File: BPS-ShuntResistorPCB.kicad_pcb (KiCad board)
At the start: 2 copper layers, 37.6 x 32.5 mm, 7 parts, among them J1 Amp_Conn

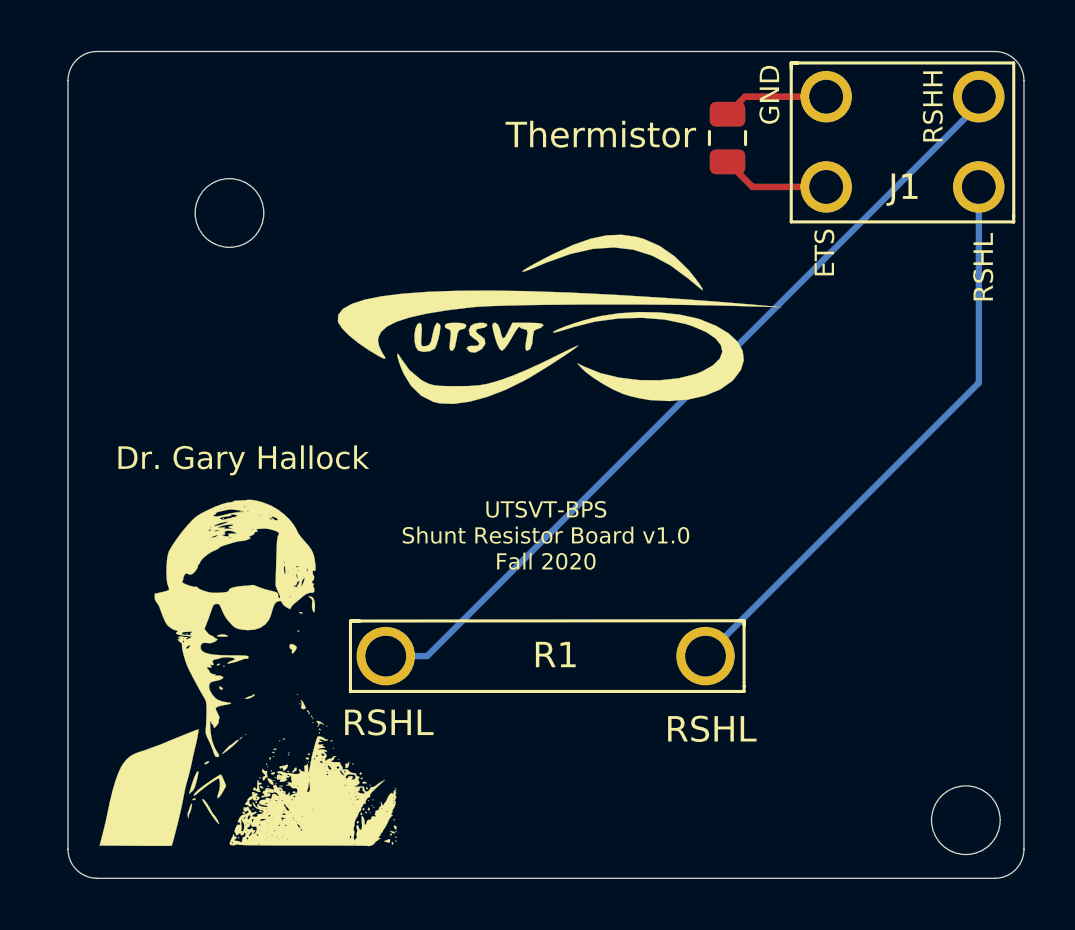
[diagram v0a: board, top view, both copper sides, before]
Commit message: fixed typo
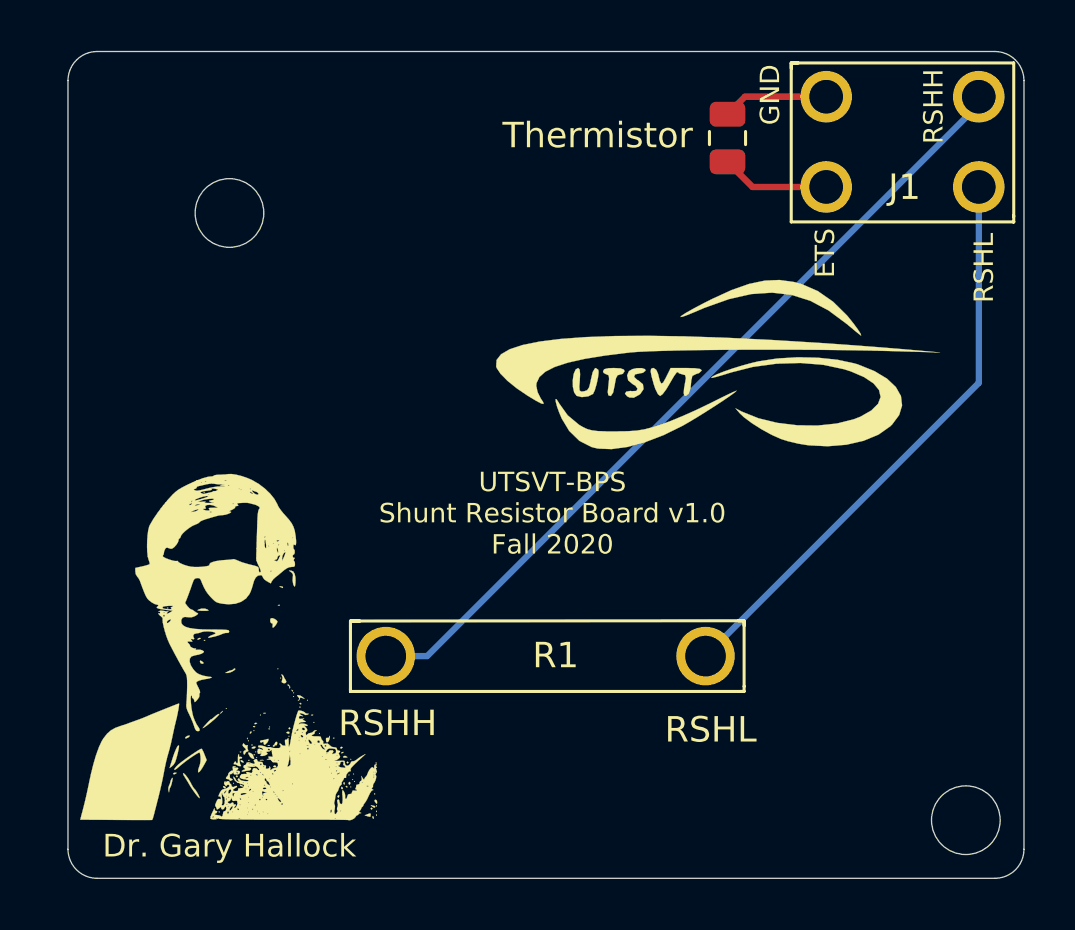
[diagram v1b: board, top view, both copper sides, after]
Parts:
- moved LOGO1 6.47 mm to (168.8, 84.7)
- moved LOGO2 1.27 mm to (149.4, 95.5)
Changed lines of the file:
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@@
     (mod_text_size 1 1)
     (mod_text_width 0.15)
-    (pad_size 2.028 2.028)
-    (pad_drill 1.328)
+    (pad_size 2.7 2.7)
+    (pad_drill 2.7)
     (pad_to_mask_clearance 0.05)
     (aux_axis_origin 0 0)
@@
       (effects (font (size 1 1) (thickness 0.15)))
     )
-    (pad 1 np_thru_hole circle (at 0 0) (size 2.7 2.7) (drill 2.7) (layers *.Cu *.Mask))
+    (pad "" np_thru_hole circle (at 0 0) (size 2.7 2.7) (drill 2.7) (layers *.Cu *.Mask))
   )
   (module UTSVT_Connectors:Power_Metal_Strip_Battery_Shunt_Resistor_4_Pin_Connector (layer F.Cu)
@@
     (tags resistor)
     (attr smd)
-    (fp_text reference Thermistor (at -0.1016 4.9784 180) (layer F.SilkS)
+    (fp_text reference Thermistor (at -0.1016 5.1054 180) (layer F.SilkS)
       (effects (font (size 1 1) (thickness 0.15)))
     )
@@
   )
   (module UTSVT_Special:Hallock_Image_Tiny (layer F.Cu)
-    (at 150.114 96.52)
+    (at 149.352 95.504)
     (fp_text reference LOGO2 (at 0 0) (layer B.SilkS) hide
       (effects (font (size 1.524 1.524) (thickness 0.3)) (justify mirror))
@@
   )
   (module UTSVT_Special:UTSVT_Logo_Symbol (layer F.Cu)
-    (at 162.56 82.931)
+    (at 168.783 84.709)
     (fp_text reference LOGO1 (at 0 0) (layer F.SilkS) hide
       (effects (font (size 1.524 1.524) (thickness 0.3)))
@@
     (arrow2b (pts (xy 139.4968 96.0374) (xy 140.083221 97.163904)))
   )
-  (gr_text RSHL (at 156.083 98.679) (layer F.SilkS)
+  (gr_text RSHH (at 156.083 98.679) (layer F.SilkS)
     (effects (font (size 1 1) (thickness 0.15)))
   )
@@
     (effects (font (size 0.762 0.762) (thickness 0.15)))
   )
-  (gr_text "UTSVT-BPS\nShunt Resistor Board v1.0\nFall 2020\n" (at 162.306 91.313) (layer F.SilkS)
-    (effects (font (size 0.635 0.635) (thickness 0.1143)))
-  )
-  (gr_text "Dr. Gary Hallock" (at 150.368 88.265) (layer F.SilkS)
-    (effects (font (size 0.889 0.889) (thickness 0.1905)))
+  (gr_text "UTSVT-BPS\nShunt Resistor Board v1.0\nFall 2020\n" (at 162.56 90.424) (layer F.SilkS)
+    (effects (font (size 0.762 0.762) (thickness 0.127)))
+  )
+  (gr_text "Dr. Gary Hallock" (at 149.86 103.505) (layer F.SilkS)
+    (effects (font (size 0.889 0.889) (thickness 0.1778)))
   )
   (gr_line (start 179.959 104.775) (end 144.653 104.775) (layer Edge.Cuts) (width 0.05))
